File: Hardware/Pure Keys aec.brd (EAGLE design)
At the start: 97.8 x 98.7 mm, 58 parts, among them IC1 TL074P, IC2 TL072P, IC5 TL074P, Q2 20MHz, T1 2N3904, U2 LM4040A50IDBZT, U3 328P

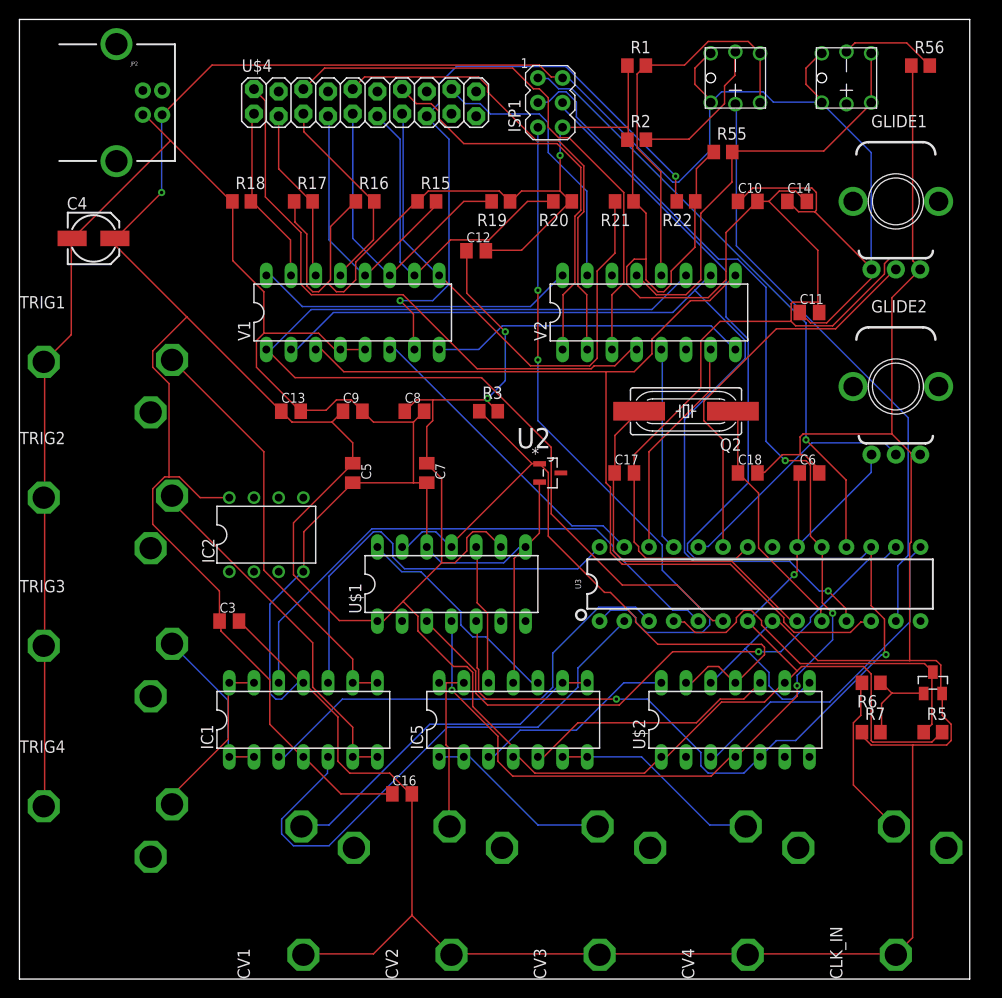
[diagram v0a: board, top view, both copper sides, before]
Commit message: Slight update
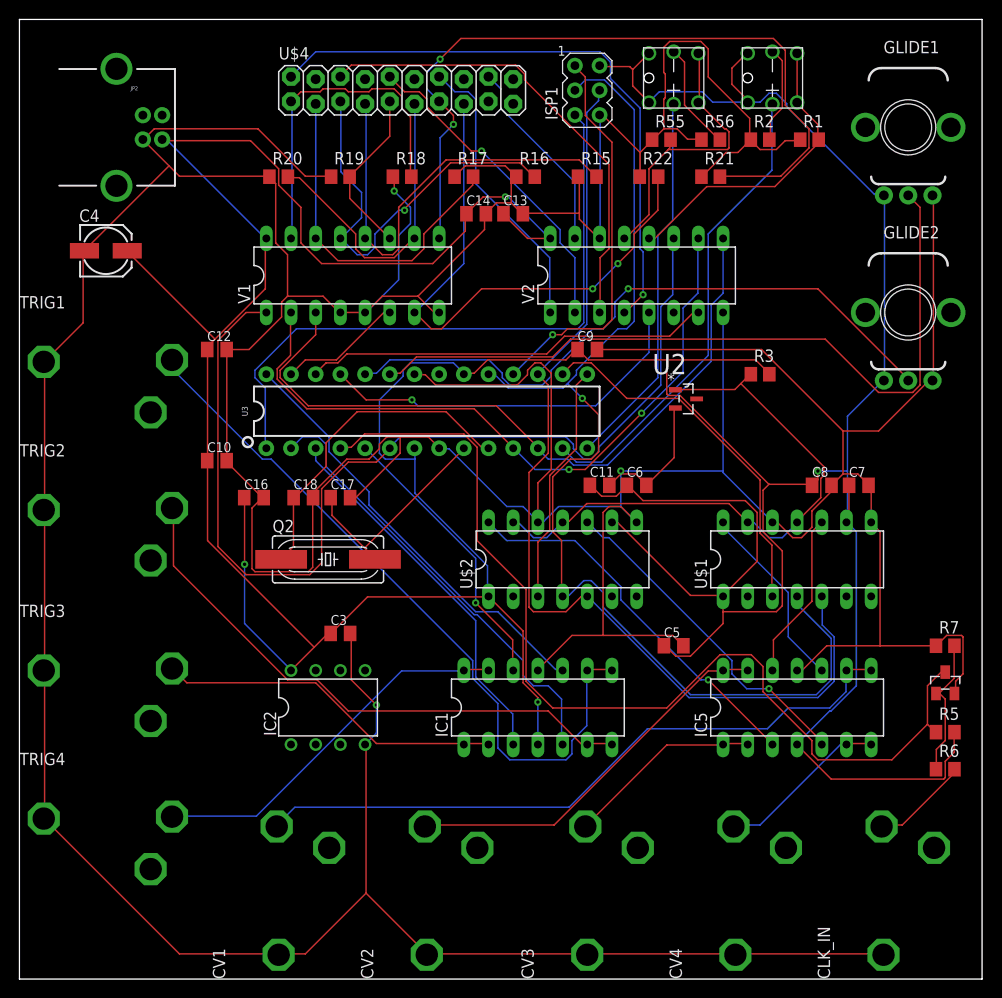
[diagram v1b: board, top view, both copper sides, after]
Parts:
- removed U$6, U$7: PB6149L-5, INSTRUO:PB6149L
- added BUT1, BUT2: PB6149L-5, INSTRUO:PB6149L
- moved C10 60.8 mm to (20.3, 53.3)
- moved C18 45.8 mm to (29.2, 49.5)
- moved C7 44.5 mm to (86.4, 50.8), turned to 0 degrees
- moved C8 42.6 mm to (82.5, 50.8)
- moved Q2 39.9 mm to (31.8, 43.2), turned to 0 degrees
- moved U3 38.6 mm to (41.9, 58.4)
- moved C5 37.5 mm to (67.3, 34.3), turned to 0 degrees
- moved U$1 35.7 mm to (80.0, 43.2)
- moved C16 34.1 mm to (24.1, 49.5)
- moved C14 33.0 mm to (47.0, 78.7)
- moved C13 30.6 mm to (50.8, 78.7)
- moved C17 29.3 mm to (33.0, 49.5)
- moved R20 29.3 mm to (26.7, 82.5), turned to 0 degrees
- moved IC5 29.2 mm to (80.0, 27.9)
- moved C12 28.5 mm to (20.3, 64.8)
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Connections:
- removed net +UB: V1.16, V2.16
- removed net -UB: V1.8, V2.8
- removed net CLK_OUT: U3.14
- removed net MK5: V2.14
- net 5V: now also BUT1.3, BUT1.4, BUT2.3, BUT2.4, V1.16, V2.16; no longer U$6.3, U$6.4, U$7.3, U$7.4
- net BUT1: now also BUT1.1, BUT1.2; no longer U$7.1, U$7.2
- net BUT2: now also BUT2.1, BUT2.2; no longer U$6.1, U$6.2
- net BUTLED1: now also BUT1.A, U3.14; no longer U$7.A
- net BUTLED2: now also BUT2.A; no longer U$6.A
- net GND: now also V1.8, V2.14, V2.8
- net N$65: now also BUT1.K; no longer U$7.K
- net N$8: now also BUT2.K; no longer U$6.K
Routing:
- net CLK_IN: track 37.9 -> 102.1 mm
- net MOSI: track 146.7 -> 103.6 mm, vias 2 -> 0
- net POT2: track 25.3 -> 67.2 mm, vias 0 -> 1
- net BUTLED1: track 0.00 -> 39.1 mm
- net POT1: track 41.2 -> 78.7 mm
- net N$7: track 35.6 -> 69.2 mm
- net +UB: track 33.1 -> 0.00 mm
- net -UB: track 32.5 -> 0.00 mm
- net N$4: track 43.5 -> 74.6 mm
- net 5V: track 476.7 -> 505.4 mm
- net TRIG4: track 57.6 -> 29.2 mm, vias 0 -> 1
- net A1OUT: track 98.3 -> 71.7 mm, vias 1 -> 2
- net A2OUT: track 98.9 -> 74.0 mm
- net T6: track 55.6 -> 79.2 mm, vias 0 -> 2
- net N$36: track 17.5 -> 40.1 mm
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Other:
- board size 97.8 x 98.7 mm -> 99 x 98.7 mm
